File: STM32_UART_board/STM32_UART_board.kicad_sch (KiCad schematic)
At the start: 21 parts, among them J1 SWD, J2 Scooter, J4 Conn_01x10, J5 Conn_01x10, SW1 SW_Push, U1 LM2574HVM-5, U3 AMS1117-3.3, U4 STM32C011J6Mx, U5 STM32C011F6Px

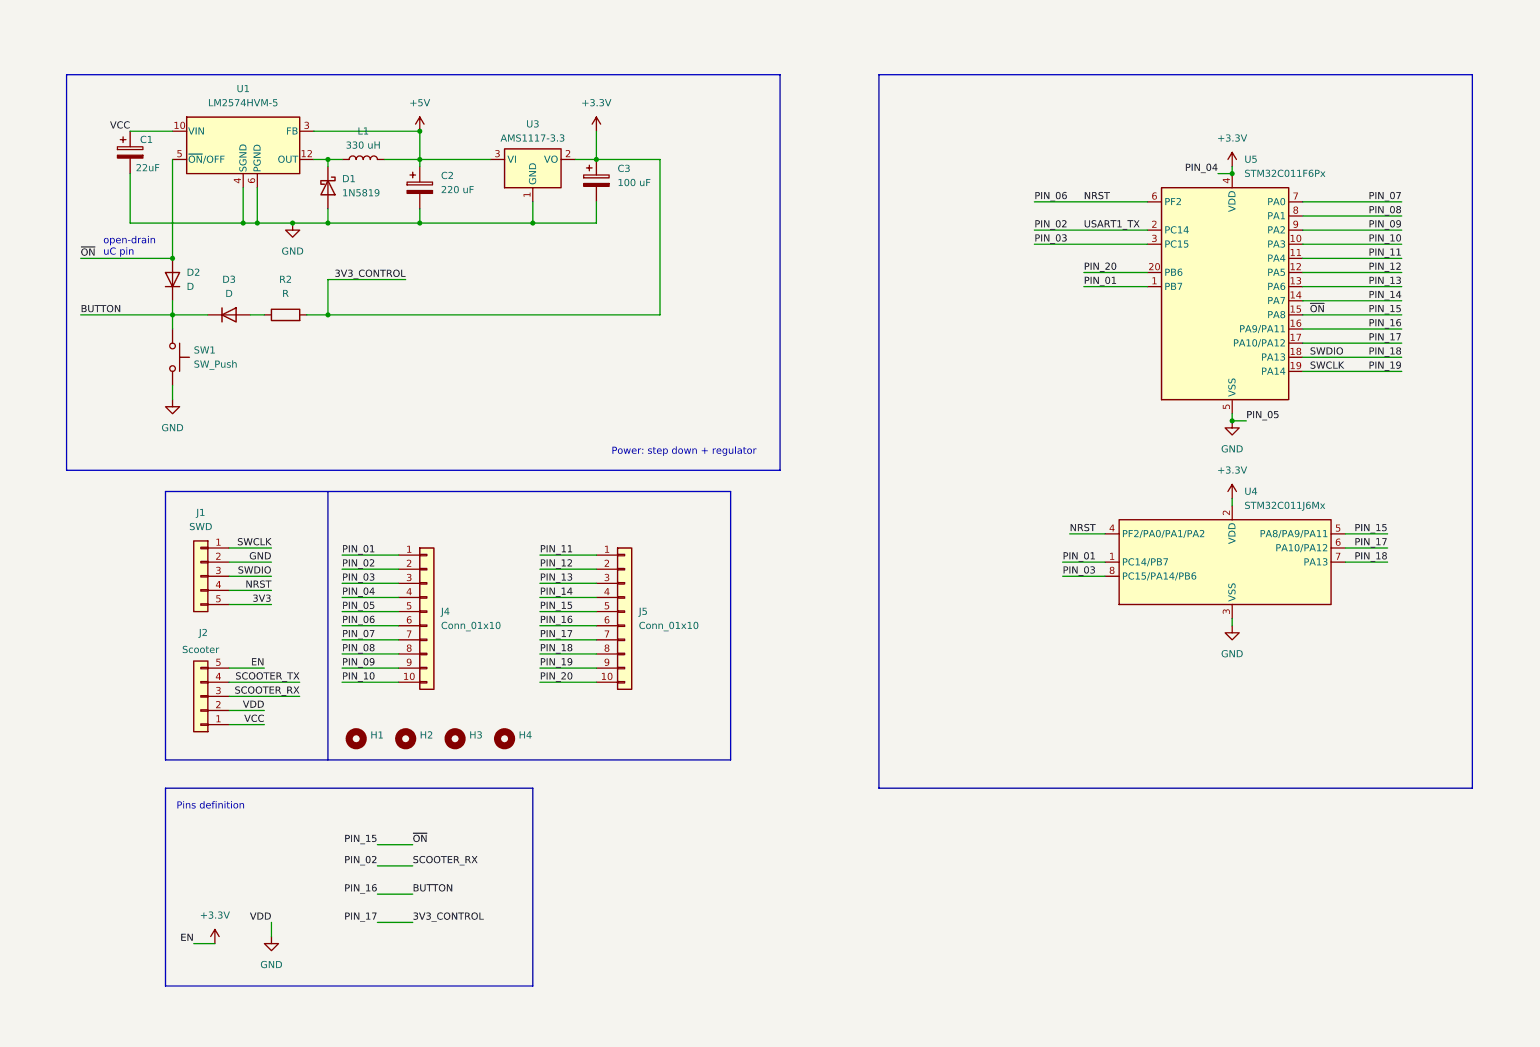
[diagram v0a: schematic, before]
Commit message: schematic mostly done
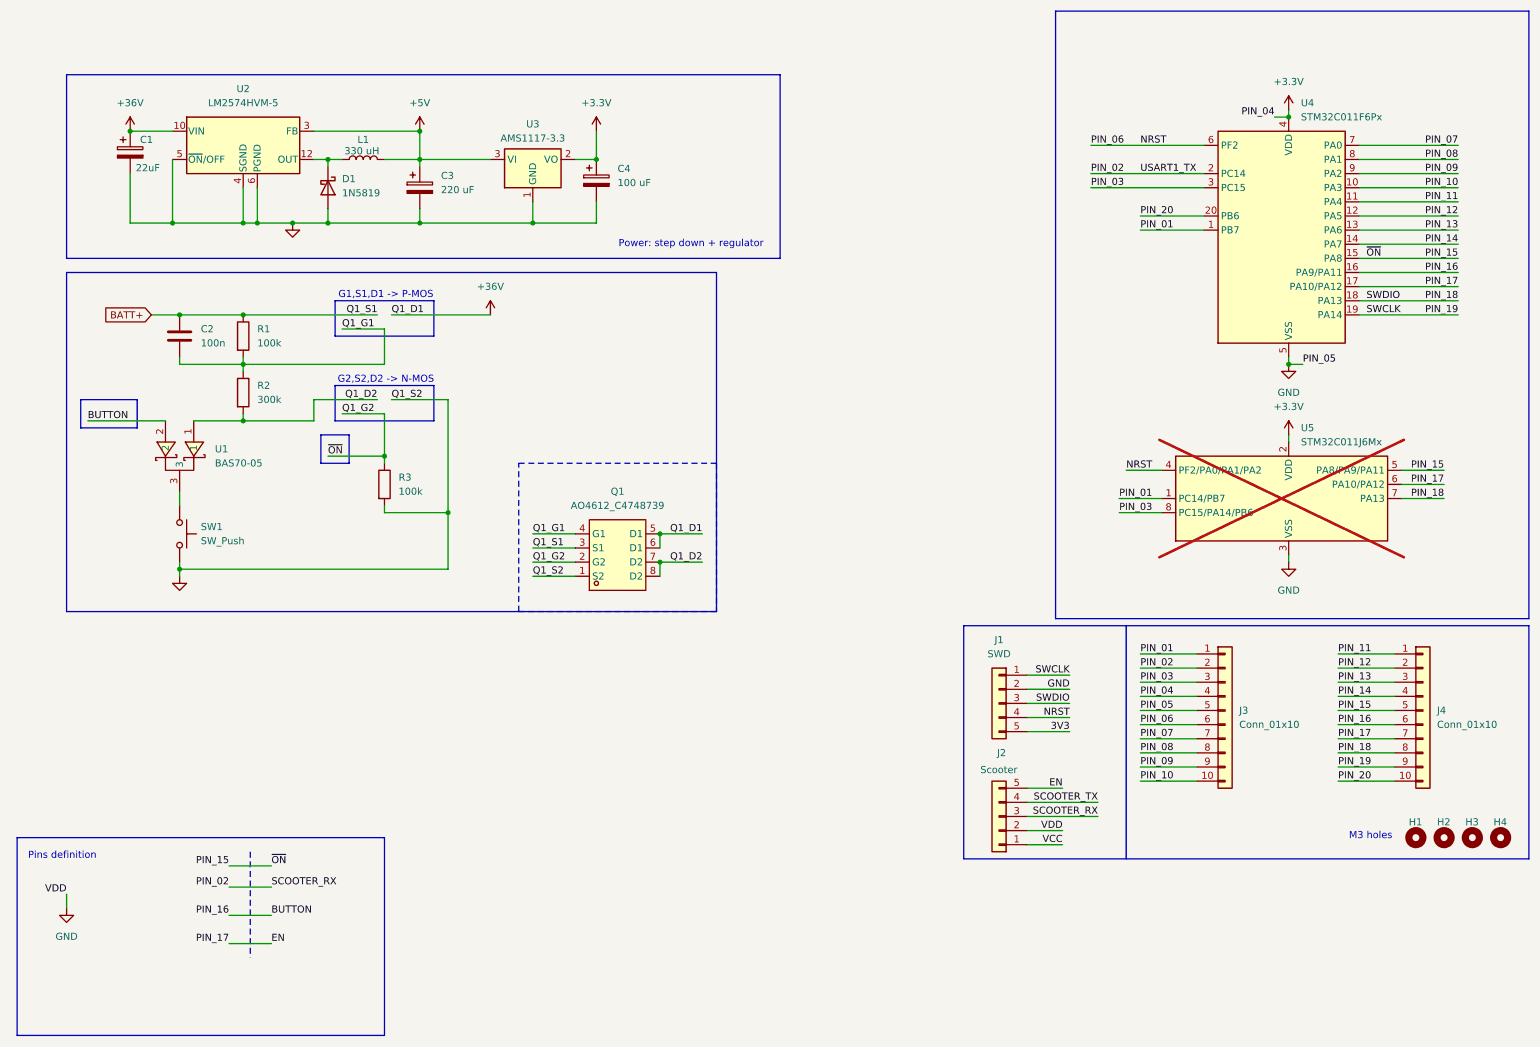
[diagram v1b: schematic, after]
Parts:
- removed D2, D3: D, symbol Device:D
- added C2: 100n, Capacitor_SMD:C_0603_1608Metric_Pad1.08x0.95mm_HandSolder, symbol Device:C
- added Q1: AO4612_C4748739, easyeda2kicad:SOIC-8_L4.9-W3.9-P1.27-LS6.0-BL-2, symbol easyeda2kicad:AO4612_C4748739
- added R1, R3: 100k, symbol Device:R
- added U1: BAS70-05, easyeda2kicad:SOT-23-3_L2.9-W1.3-P1.90-LS2.4-BR, symbol easyeda2kicad:BAS70-05_C7461133
- H1, H2, H3, H4: value ~ -> MountingHole; footprint MountingHole:MountingHole_3.2mm_M3_DIN965_Pad -> MountingHole:MountingHole_3.2mm_M3; now in the parts list
- R2: value R -> 300k; footprint Resistor_SMD:R_0603_1608Metric -> (none)
- SW1: footprint Connector_PinHeader_2.54mm:PinHeader_1x02_P2.54mm_Vertical -> (none)
- U5: renamed from U4; now not fitted; now left out of the parts list
- renumbered C2 to C3, C3 to C4, J4 to J3, J5 to J4, U1 to U2, U5 to U4
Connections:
- net +3.3V: no longer J2.5 (Pin_5), J4.7 (Pin_7), R2.2, U4.17 (PA10/PA12), U5.6 (PA10/PA12)
- net BUTTON: now also U1.2; no longer SW1.1
- net GND: now also U2.5 (~{ON}/OFF), Q1.1 (S2), R3.2
- net PIN_15: now also Q1.2 (G2), R3.1; no longer U2.5 (~{ON}/OFF)
- net VCC: no longer C1.1, U2.10 (VIN)
- net Q1_G1: now reaches R2.1
- net Q1_G1: now also C2.2, Q1.4 (G1), R1.2
- new net: SW1.1, U1.3
- new net +36V: C1.1, Q1.5 (D1), Q1.6 (D1), U2.10 (VIN)
- new net BATT+: C2.1, Q1.3 (S1), R1.1
- new net EN: J2.5 (Pin_5), J4.7 (Pin_7), U4.17 (PA10/PA12), U5.6 (PA10/PA12)
- new net Q1_D2: Q1.7 (D2), Q1.8 (D2), R2.2, U1.1
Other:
- note added: "G1,S1,D1 -> P-MOS"
- note added: "G2,S2,D2 -> N-MOS"
- note added: "M3 holes"
- note removed: "open-drain uC pin"
- moved on the sheet: J1, J2, J3, J4, U4
